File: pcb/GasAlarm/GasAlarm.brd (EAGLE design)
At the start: 100 x 80 mm, 12 parts, among them IC1 ULN2003AN

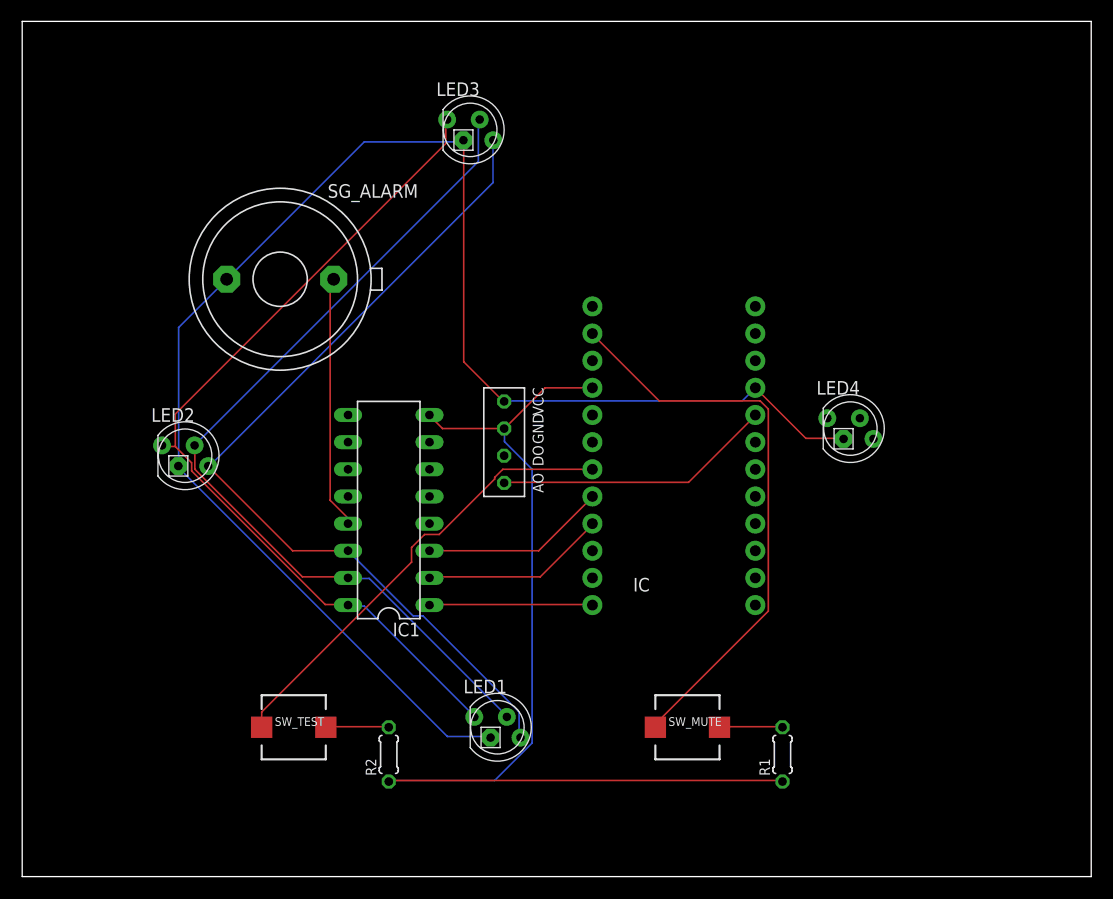
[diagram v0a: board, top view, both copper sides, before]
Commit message: pcb完成
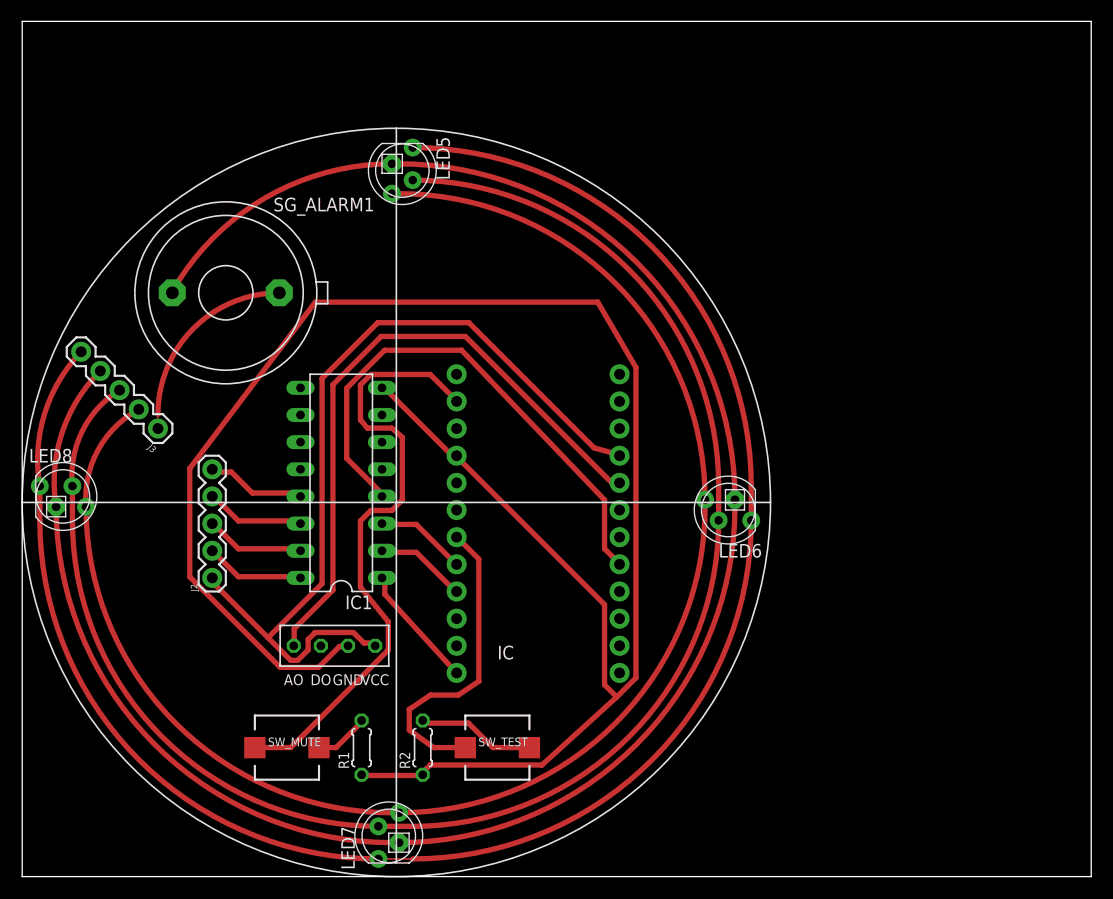
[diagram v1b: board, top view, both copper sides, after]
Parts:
- removed LED1, LED2, LED3, LED4: RGBLED_CA-5MM, adafruit:LED5MMRGB
- removed SG_ALARM: F/EE17P, buzzer:F/EE17P
- removed U$1: MQ-6, GasAlarm:DIP4-MQ_6
- added J2, J3: (no value), SparkFun-Connectors:1X05
- added LED5, LED6, LED7, LED8: RGBLED_CA-5MM, adafruit:LED5MMRGB
- added MQ6: MQ-6, GasAlarm:DIP4-MQ_6
- added SG_ALARM1: F/EE17P, buzzer:F/EE17P
- moved R1 39.4 mm to (31.8, 12.1)
- moved SW_MUTE 37.5 mm to (24.8, 12.1)
- moved SW_TEST 19.1 mm to (44.5, 12.1)
- moved IC 14.2 mm to (48.3, 34.3)
- moved IC1 5.12 mm to (29.8, 36.8)
- moved R2 3.24 mm to (37.5, 12.1)
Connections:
- new net N$14: IC.17, IC1.4
- new net N$19: J3.5, LED5.1, LED6.1, LED7.1, LED8.1
- new net N$20: J3.4, LED5.2, LED6.2, LED7.2, LED8.2, SG_ALARM1.1
- new net N$21: J3.3, LED5.3, LED6.3, LED7.3, LED8.3
- new net N$22: J3.2, LED5.4, LED6.4, LED7.4, LED8.4
- new net N$23: J3.1, SG_ALARM1.2
- net GND: now also MQ6.3; no longer U$1.3
- net N$1: now also J2.2; no longer LED1.1, LED2.1, LED3.1
- net N$12: now also MQ6.1; no longer U$1.1
- net N$2: now also J2.3; no longer LED1.3, LED2.3, LED3.3
- net N$3: now also J2.4; no longer LED1.4, LED2.4, LED3.4
- net N$4: now also J2.5; no longer SG_ALARM.2
- net VCC: now also J2.1, MQ6.4; no longer LED1.2, LED2.2, LED3.2, LED4.2, SG_ALARM.1, U$1.4
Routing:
- net N$20: track 0.00 -> 172.8 mm
- net N$19: track 0.00 -> 157.1 mm
- net N$21: track 0.00 -> 141.1 mm
- net N$22: track 0.00 -> 133.8 mm
- net GND: track 99.8 -> 179.2 mm
- net N$2: track 82.7 -> 9.27 mm
- net N$3: track 82.7 -> 9.30 mm
- net N$1: track 81.5 -> 9.28 mm
- net VCC: track 147.0 -> 82.4 mm
- net N$14: track 0.00 -> 49.7 mm
- net N$12: track 26.2 -> 60.3 mm
- net N$23: track 0.00 -> 17.4 mm
- net N$4: track 23.7 -> 9.36 mm
- net N$5: track 42.7 -> 29.4 mm
- net N$7: track 17.5 -> 8.52 mm
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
